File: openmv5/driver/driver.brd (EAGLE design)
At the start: 35.6 x 26.7 mm, 87 parts, among them IC1 TPS613222ADBVR, IC2 AP64060WU-7, IC3 LM321LVIDCKR, IC4 74LVC1G07GW,125, IC5 DRV8876RGTR, IC6 DRV8876RGTR, J1 OPENMV5-TOP, J2 1771088, Q1 BUK6D120-60PX, U1 74LVC1G17SE-7

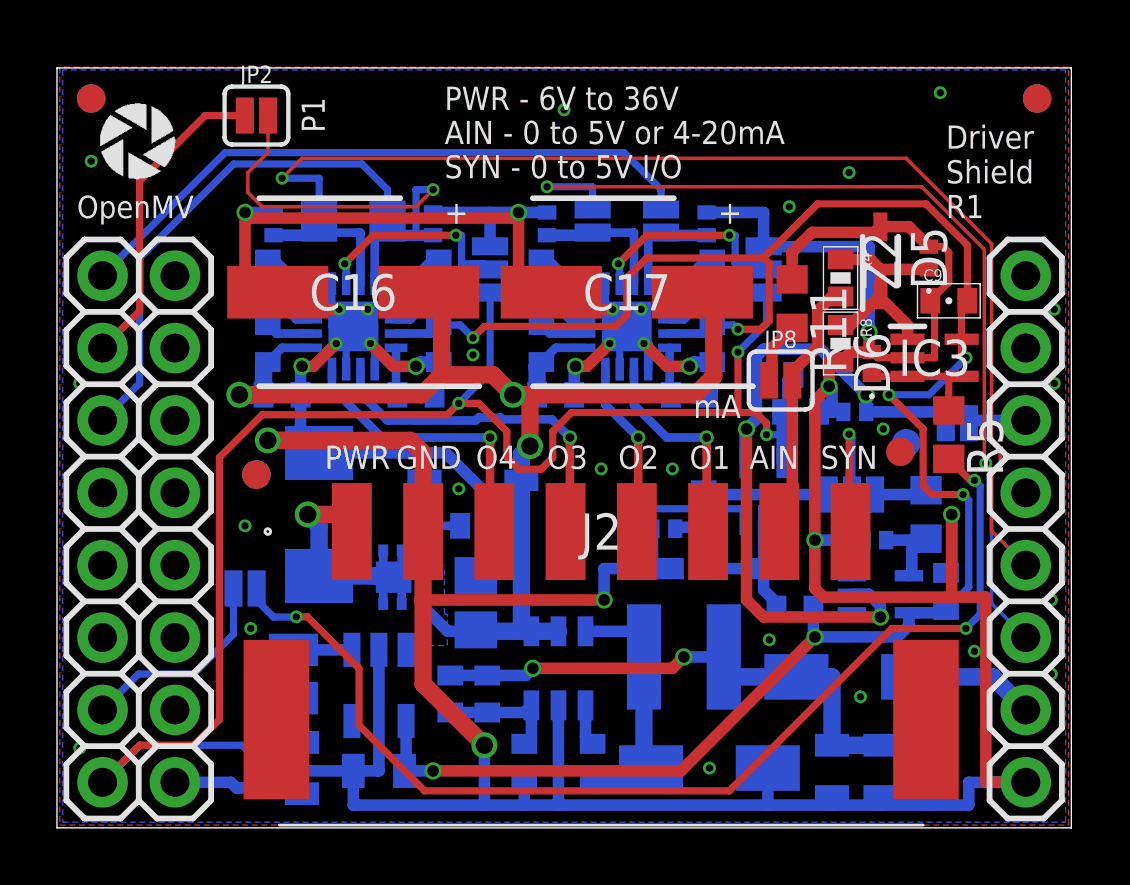
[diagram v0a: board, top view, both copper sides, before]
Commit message: Fix placement
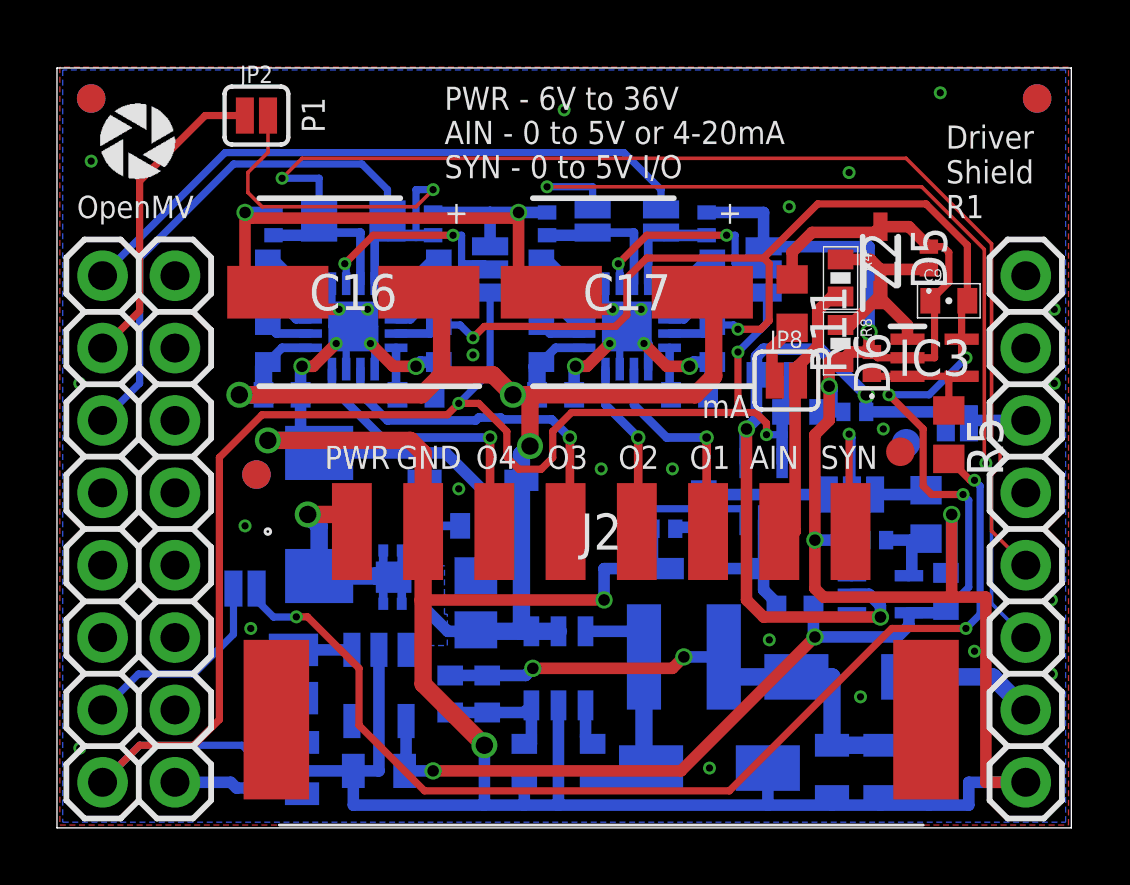
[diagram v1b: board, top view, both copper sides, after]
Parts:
- moved JP8 0.20 mm to (25.6, 15.7)
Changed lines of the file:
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@@
 <text x="29" y="13" size="0.8128" layer="22" font="vector" ratio="22" rot="MR0">O</text>
 <text x="27.3" y="13" size="0.8128" layer="22" font="vector" ratio="22" rot="MR0">I</text>
-<text x="24" y="15.2" size="0.8128" layer="21" font="vector" ratio="22" rot="R180">mA</text>
+<text x="24.3" y="15.2" size="0.8128" layer="21" font="vector" ratio="22" rot="R180">mA</text>
 <text x="13.6" y="25.2" size="0.8128" layer="21" font="vector" ratio="20">PWR - 6V to 36V </text>
 <text x="13.6" y="24" size="0.8128" layer="21" font="vector" ratio="20">AIN - 0 to 5V or 4-20mA</text>
@@
 <attribute name="VALUE" x="30.8" y="16.5" size="1.27" layer="27" align="center"/>
 </element>
-<element name="JP8" library="SparkFun-Jumpers" library_urn="urn:adsk.eagle:library:528" package="SMT-JUMPER_2_NO_SILK" package3d_urn="urn:adsk.eagle:package:39279/1" value="JUMPER-SMT_2_NO_SILK" x="25.4" y="15.7" smashed="yes">
-<attribute name="NAME" x="25.4" y="16.843" size="0.6096" layer="25" font="vector" ratio="20" align="bottom-center"/>
-<attribute name="VALUE" x="25.4" y="14.557" size="0.6096" layer="27" font="vector" ratio="20" align="top-center"/>
+<element name="JP8" library="SparkFun-Jumpers" library_urn="urn:adsk.eagle:library:528" package="SMT-JUMPER_2_NO_SILK" package3d_urn="urn:adsk.eagle:package:39279/1" value="JUMPER-SMT_2_NO_SILK" x="25.6" y="15.7" smashed="yes">
+<attribute name="NAME" x="25.6" y="16.843" size="0.6096" layer="25" font="vector" ratio="20" align="bottom-center"/>
+<attribute name="VALUE" x="25.6" y="14.557" size="0.6096" layer="27" font="vector" ratio="20" align="top-center"/>
 </element>
 <element name="C9" library="sfe" package="0402-CAP" value="0.1uF" x="31.3" y="18.5" smashed="yes">
@@
 <via x="27.1" y="15.5" extent="1-16" drill="0.4064"/>
 <wire x1="27.2" y1="14.6" x2="26.75" y2="14.6" width="0.4064" layer="16"/>
-<wire x1="27.1" y1="15.5" x2="26.6" y2="15" width="0.4064" layer="1"/>
-<wire x1="26.6" y1="15" x2="26.6" y2="10.1" width="0.4064" layer="1"/>
+<wire x1="27.1" y1="15.5" x2="27.1" y2="14.3" width="0.4064" layer="1"/>
+<wire x1="27.1" y1="14.3" x2="26.6" y2="13.8" width="0.4064" layer="1"/>
+<wire x1="26.6" y1="13.8" x2="26.6" y2="10.1" width="0.4064" layer="1"/>
 <contactref element="D5" pad="2"/>
 <contactref element="R8" pad="2"/>
@@
 <contactref element="R4" pad="2"/>
 <contactref element="JP8" pad="2"/>
-<wire x1="25.8064" y1="15.7" x2="25.8064" y2="10.4" width="0.4064" layer="1"/>
-<wire x1="25.8064" y1="10.4" x2="25.35" y2="10.4" width="0.4064" layer="1"/>
-<wire x1="25.8064" y1="15.7" x2="25.8064" y2="16.0064" width="0.4064" layer="1"/>
-<wire x1="26.7" y1="16.9" x2="25.8064" y2="16.0064" width="0.4064" layer="1"/>
+<wire x1="26.0064" y1="15.7" x2="25.9064" y2="15.6" width="0.4064" layer="1"/>
+<wire x1="25.9064" y1="15.6" x2="25.9064" y2="10.4" width="0.4064" layer="1"/>
+<wire x1="25.9064" y1="10.4" x2="25.35" y2="10.4" width="0.4064" layer="1"/>
+<wire x1="26.0064" y1="15.7" x2="26.0064" y2="16.2064" width="0.4064" layer="1"/>
+<wire x1="26.7" y1="16.9" x2="26.0064" y2="16.2064" width="0.4064" layer="1"/>
 <wire x1="27.5" y1="18.65" x2="27.2" y2="18.65" width="0.4064" layer="1"/>
 <wire x1="27.2" y1="18.65" x2="26.7" y2="18.15" width="0.4064" layer="1"/>
@@
 <contactref element="JP8" pad="1"/>
 <contactref element="R11" pad="2"/>
-<wire x1="24.9936" y1="15.7" x2="25.0936" y2="15.8" width="0.4064" layer="1"/>
+<wire x1="25.1936" y1="15.7" x2="25.0936" y2="15.8" width="0.4064" layer="1"/>
 <wire x1="25.0936" y1="16.8436" x2="25.0936" y2="15.8" width="0.4064" layer="1"/>
 <wire x1="25.8" y1="17.55" x2="25.0936" y2="16.8436" width="0.4064" layer="1"/>
@@
 <via x="19.7" y="19.8" extent="1-16" drill="0.254"/>
 <wire x1="19.7" y1="19.8" x2="20.7" y2="20.8" width="0.254" layer="1"/>
-<wire x1="20.7" y1="20.8" x2="23.6" y2="20.8" width="0.254" layer="1"/>
-<via x="23.6" y="20.8" extent="1-16" drill="0.254"/>
-<wire x1="23.6" y1="20.8" x2="23.8" y2="20.8" width="0.254" layer="16"/>
+<wire x1="20.7" y1="20.8" x2="23.5" y2="20.8" width="0.254" layer="1"/>
+<via x="23.5" y="20.8" extent="1-16" drill="0.254"/>
+<wire x1="23.5" y1="20.8" x2="23.8" y2="20.8" width="0.254" layer="16"/>
 <wire x1="24.6" y1="19.8" x2="23.8" y2="19.8" width="0.254" layer="16"/>
 <wire x1="24.6" y1="19.8" x2="24.8" y2="19.6" width="0.254" layer="16"/>
@@
 <via x="10.1" y="19.8" extent="1-16" drill="0.254"/>
 <wire x1="10.1" y1="19.8" x2="11.1" y2="20.8" width="0.254" layer="1"/>
-<wire x1="11.1" y1="20.8" x2="14" y2="20.8" width="0.254" layer="1"/>
-<via x="14" y="20.8" extent="1-16" drill="0.254"/>
-<wire x1="14" y1="20.8" x2="14.2" y2="20.8" width="0.254" layer="16"/>
+<wire x1="11.1" y1="20.8" x2="13.9" y2="20.8" width="0.254" layer="1"/>
+<via x="13.9" y="20.8" extent="1-16" drill="0.254"/>
+<wire x1="13.9" y1="20.8" x2="14.2" y2="20.8" width="0.254" layer="16"/>
 <wire x1="15" y1="19.8" x2="14.2" y2="19.8" width="0.254" layer="16"/>
 <wire x1="15" y1="19.8" x2="15.2" y2="19.6" width="0.254" layer="16"/>
